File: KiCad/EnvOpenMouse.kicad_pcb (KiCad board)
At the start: 2 copper layers, 34.5 x 42.7 mm, 49 parts, among them J1 SKRKAEE020, J2 SKRKAEE020, J3 Conn_01x03_Male, U1 TCR2EF19, U2 LM3671MF 3.3, U3 PMW3360DM-T2QU, U4 RP2040, Y1 Crystal 3225 12MHz

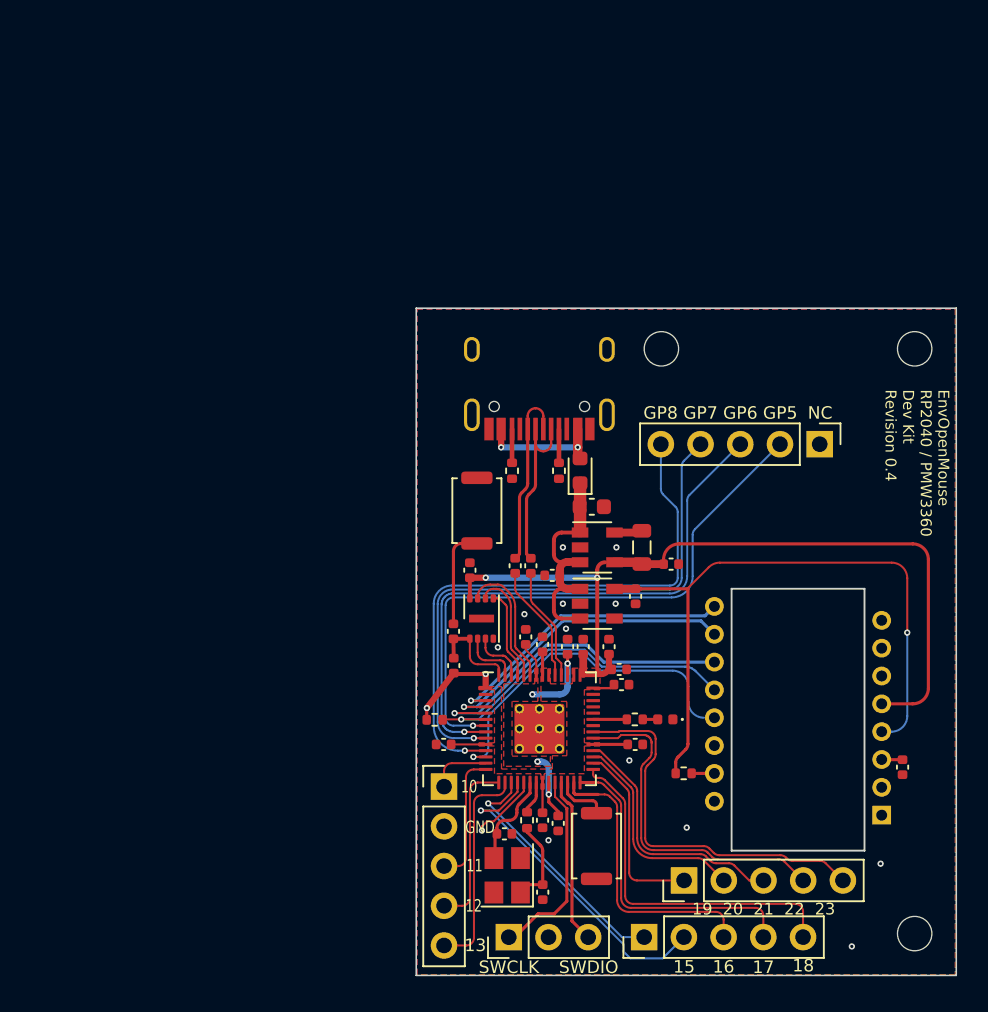
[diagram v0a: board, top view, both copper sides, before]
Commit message: decided to overhaul this project a bit
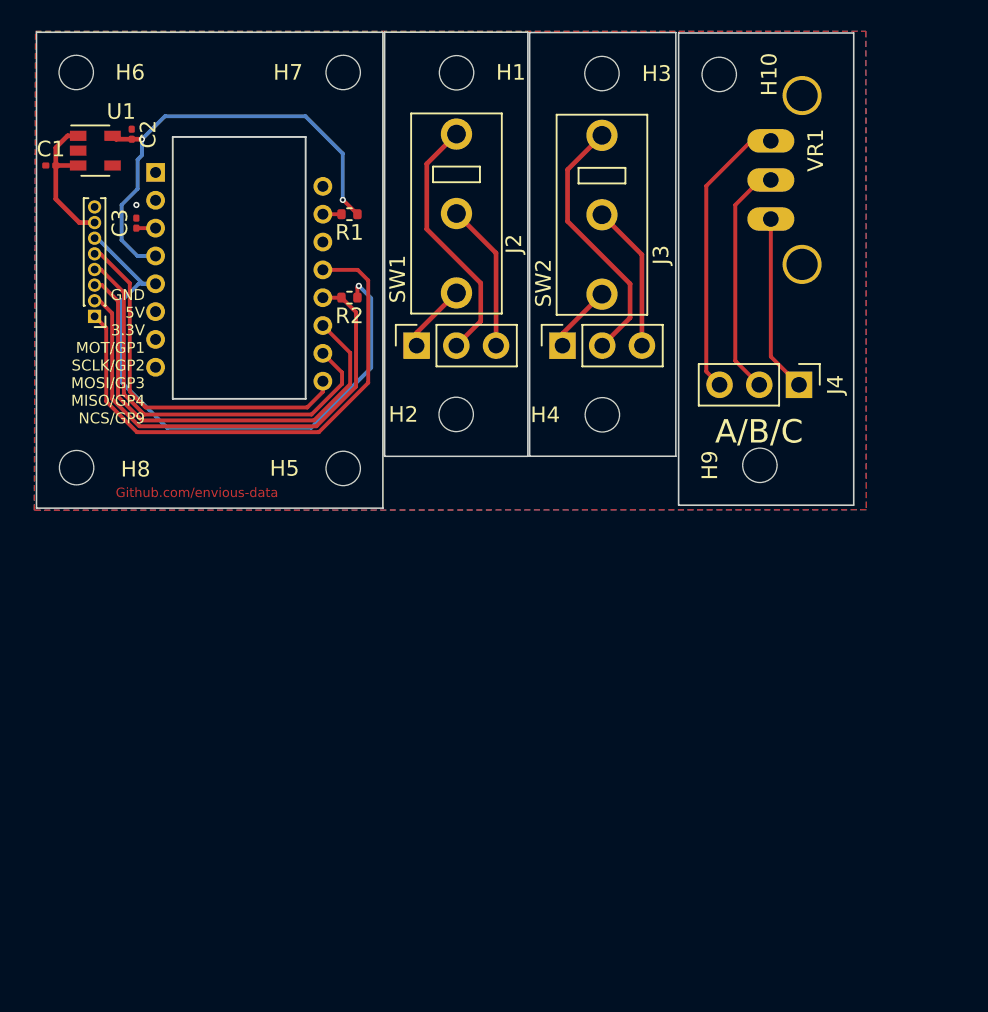
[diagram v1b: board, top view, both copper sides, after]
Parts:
- removed C10, C11, C12, C13, C14, C17, C6, C7, C8, C9: 100nf 0402, Capacitor_SMD:C_0402_1005Metric
- removed C15, C16: 1uf 0402, Capacitor_SMD:C_0402_1005Metric
- removed C18, C19: 22pf 0402, Capacitor_SMD:C_0402_1005Metric
- removed C4: 10uf 0402, Capacitor_SMD:C_0402_1005Metric
- removed C5: 4.7uf 0402, Capacitor_SMD:C_0402_1005Metric
- removed D1: 1n4002 0603, Diode_SMD:D_0603_1608Metric
- removed D2: LED 0402 YELLOW, LED_SMD:LED_0402_1005Metric
- removed FLASH1: W25Q16FWUXIE, Package_SON:SON-8-1EP_3x2mm_P0.5mm_EP1.4x1.6mm
- removed GPIOA1, GPIOA2, SCRL1: Rotary_Encoder_Switch, Connector_PinHeader_2.54mm:PinHeader_1x05_P2.54mm_Vertical
- removed GPIOA3: GPIOs, Connector_PinHeader_2.54mm:PinHeader_1x05_P2.54mm_Vertical
- removed L1: INDUCTOR 2.2uH 0805, Inductor_SMD:L_0805_2012Metric
- removed R10: 1K 0402, Resistor_SMD:R_0402_1005Metric
- removed R3: 10K 0402, Resistor_SMD:R_0402_1005Metric
- removed R4: 5.1K, Resistor_SMD:R_0402_1005Metric
- removed R5: 10K 0402, Capacitor_SMD:C_0402_1005Metric
- removed R6, R7: 27Ohms 0402 Resistor, Capacitor_SMD:C_0402_1005Metric
- removed R8: 1k 0402 Resistor, Capacitor_SMD:C_0402_1005Metric
- removed R9: 470 ohm resistor, Resistor_SMD:R_0402_1005Metric
- removed U3: PMW3360DM-T2QU, local:DIP-16_W10.16mm
- removed U4: RP2040, env:RP2040-QFN-56
- removed Y1: Crystal 3225 12MHz, Crystal:Crystal_SMD_3225-4Pin_3.2x2.5mm
- removed e1: TYPE-C-31-M-12, Type-C:HRO-TYPE-C-31-M-12-Assembly
- added H10: MountingHole_Pad, MountingHole:MountingHole_2.2mm_M2, F.Cu at (57.5, 15.1)
- added H3: MountingHole_Pad, MountingHole:MountingHole_2.2mm_M2, F.Cu at (50.0, 15.0)
- added H5: MountingHole_Pad, MountingHole:MountingHole_2.2mm_M2, F.Cu at (33.5, 40.2)
- added H6: MountingHole_Pad, MountingHole:MountingHole_2.2mm_M2, F.Cu at (16.4, 14.9)
- added H7: MountingHole_Pad, MountingHole:MountingHole_2.2mm_M2, F.Cu at (33.5, 14.9)
- added H8: MountingHole_Pad, MountingHole:MountingHole_2.2mm_M2, F.Cu at (16.4, 40.2)
- added H9: MountingHole_Pad, MountingHole:MountingHole_2.2mm_M2, F.Cu at (60.1, 40.0)
- added J4: Conn_01x03, Connector_PinHeader_2.54mm:PinHeader_1x03_P2.54mm_Vertical, F.Cu at (62.6, 34.9)
- added SW1: SW_Push_SPDT, MouseSwitch:MouseSwitch, F.Cu at (40.7, 23.9)
- added SW2: SW_Push_SPDT, MouseSwitch:MouseSwitch, F.Cu at (50.0, 24.0)
- added VR1: EC10E1220501, EC10E1220501:TRIM_EC10E1220501, F.Cu at (60.8, 21.8)
- C1: value 10uf 0603 6.3V -> 0.1uf 0402; footprint Capacitor_SMD:C_0603_1608Metric -> Capacitor_SMD:C_0201_0603Metric
- C2: value 0.1uf 0402 -> 1uf 0402; footprint Capacitor_SMD:C_0402_1005Metric -> Capacitor_SMD:C_0201_0603Metric
- C3: value 1uf 0402 -> 4.7uf 0402; footprint Capacitor_SMD:C_0402_1005Metric -> Capacitor_SMD:C_0201_0603Metric
- H1, H2, H4: value MountingHole -> MountingHole_Pad
- J1: value SKRKAEE020 -> Conn_01x08; footprint Button_Switch_SMD:SW_Push_SPST_NO_Alps_SKRK -> Connector_PinHeader_1.00mm:PinHeader_1x08_P1.00mm_Vertical
- J2: value SKRKAEE020 -> Conn_01x03; footprint Button_Switch_SMD:SW_Push_SPST_NO_Alps_SKRK -> Connector_PinSocket_2.54mm:PinSocket_1x03_P2.54mm_Vertical
- J3: value Conn_01x03_Male -> Conn_01x03; footprint Connector_PinHeader_2.54mm:PinHeader_1x03_P2.54mm_Vertical -> Connector_PinSocket_2.54mm:PinSocket_1x03_P2.54mm_Vertical
- R2: value 5.1K -> 10K 0402
- U2: value LM3671MF 3.3 -> PMW3360DM-T2QU; footprint Package_TO_SOT_SMD:SOT-23-5 -> local:DIP-16_W10.16mm
- moved U1 43.2 mm to (17.6, 19.9)
- moved R1 41.7 mm to (33.9, 24.0), turned to 180 degrees
- moved C1 40.9 mm to (14.8, 20.9)
- moved C3 39.9 mm to (20.2, 24.6)
- moved C2 39.0 mm to (19.9, 18.9), turned to -90 degrees
- moved H4 38.7 mm to (50.0, 36.8)
- moved J3 38.0 mm to (47.5, 32.4)
- moved U2 37.2 mm to (22.6, 19.8)
- moved H1 34.2 mm to (40.7, 14.9)
- moved J2 34.0 mm to (38.1, 32.4), turned to 90 degrees
- moved J1 27.4 mm to (17.6, 30.5), turned to 180 degrees
- moved R2 17.4 mm to (33.9, 29.3), turned to 180 degrees
- moved H2 13.8 mm to (40.7, 36.8)
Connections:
- C1 pad 1: +5V -> GND
- C1 pad 2: GND -> +5V
- C2 pad 2: +5V -> +1V8
- C3 pad 1: GND -> Net-(C3-Pad1)
- C3 pad 2: +1V8 -> GND
- J1 pad 1: /~{USB_BOOT} -> NCS/GPIO9
- J1 pad 2: GND -> MISO/GPIO4
- J2 pad 1: /RUN -> Net-(J2-Pad1)
- J2 pad 2: GND -> Net-(J2-Pad2)
- J3 pad 1: /SWCLK -> Net-(J3-Pad1)
- J3 pad 2: GND -> Net-(J3-Pad2)
- J3 pad 3: /SWD -> Net-(J3-Pad3)
- R2 pad 1: GND -> +3V3
- R2 pad 2: Net-(R2-Pad2) -> MISO/GPIO4
- U2 pad 1: +5V -> unconnected-(U2-Pad1)
- U2 pad 2: GND -> unconnected-(U2-Pad2)
- U2 pad 3: +5V -> Net-(C3-Pad1)
- U2 pad 4: +3V3 -> +1V8
- U2 pad 5: Net-(L1-Pad1) -> +3V3
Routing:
- net /GPIO5: track 37.6 -> 0.00 mm, vias 1 -> 0
- net /GPIO8: track 37.4 -> 0.00 mm, vias 1 -> 0
- net /GPIO6: track 37.1 -> 0.00 mm, vias 1 -> 0
- net /GPIO7: track 36.7 -> 0.00 mm, vias 1 -> 0
- net NCS/GPIO9: track 0.00 -> 34.4 mm
- net MISO/GPIO4: track 0.00 -> 31.6 mm
- net +3V3: track 69.6 -> 38.0 mm, vias 4 -> 1
- net MOSI/GPIO3: track 0.00 -> 28.9 mm
- net SCLK/GPIO2: track 0.00 -> 26.7 mm
- net /GPIO23: track 24.6 -> 0.00 mm
- net MOTION/GPIO1: track 0.00 -> 23.8 mm
- net /GPIO18: track 22.7 -> 0.00 mm
- net NCS: track 22.1 -> 0.00 mm, vias 1 -> 0
- net /GPIO22: track 21.9 -> 0.00 mm
- net MISO: track 21.8 -> 0.00 mm, vias 1 -> 0
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- removed copper zone on F.Cu, net +1V1
- removed copper zone on F.Cu, net +3V3
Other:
- board size 34.5 x 42.7 mm -> 52.3 x 30.4 mm
- board text added: "A/B/C"
- board text added: "GND 5V 3.3V MOT/GP1 SCLK/GP2 MOSI/GP3 MISO/GP4 NCS/GP9"
- board text added: "Github.com/envious-data"
- board text removed: "10"
- board text removed: "11"
- board text removed: "12"
- board text removed: "13"
- board text removed: "15"
- board text removed: "16"
- board text removed: "17"
- board text removed: "18"
- board text removed: "19 20 21 22 23"
- board text removed: "EnvOpenMouse RP2040 / PMW3360 Dev Kit Revision 0.4"
- board text removed: "GND"
- board text removed: "GP5"
- board text removed: "GP6"
- board text removed: "GP7"
- board text removed: "GP8"
- board text removed: "NC"
- board text removed: "SWCLK"
- board text removed: "SWDIO"
